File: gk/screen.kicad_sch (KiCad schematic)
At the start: 8 parts, among them J3 Conn_02x27_Top_Bottom, U5 PT4110E89E

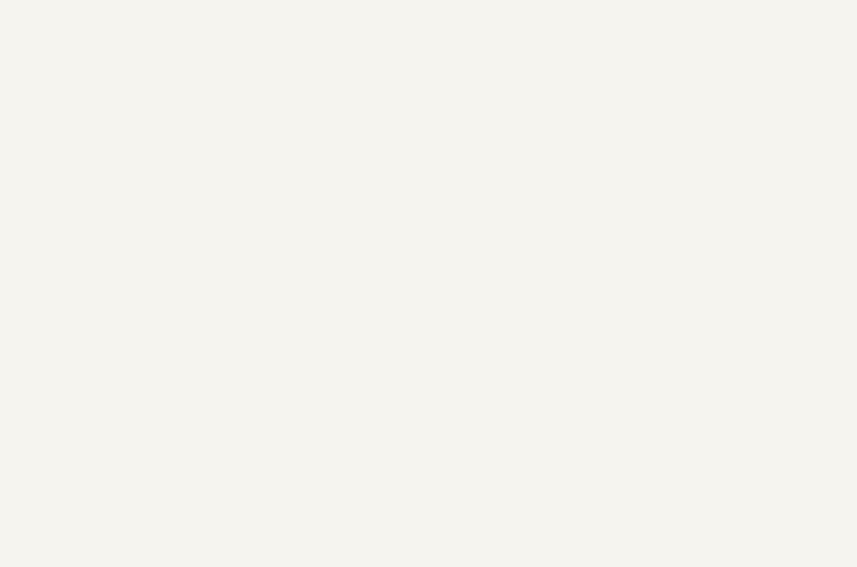
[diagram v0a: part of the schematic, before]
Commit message: Update pcb
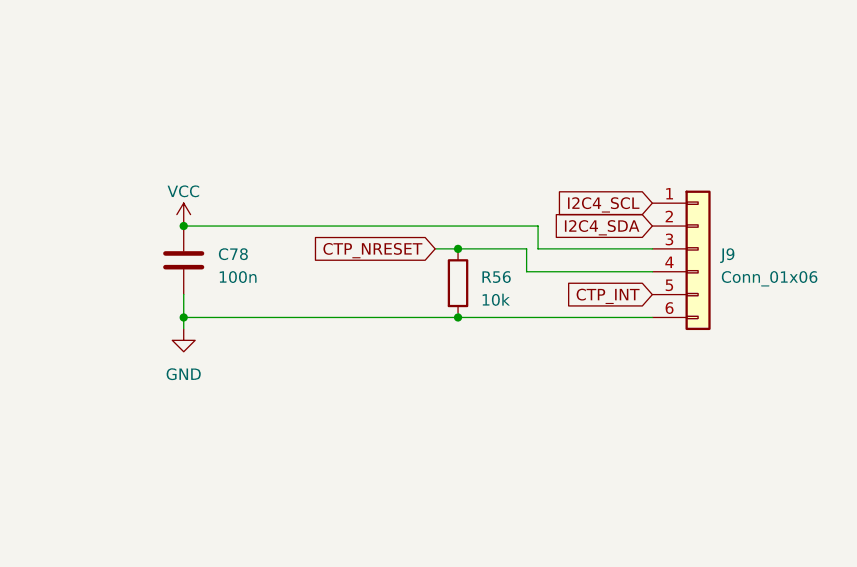
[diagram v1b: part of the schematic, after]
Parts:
- added C78: 100n, Capacitor_SMD:C_0603_1608Metric, symbol Device:C
- added J9: Conn_01x06, Connector_FFC-FPC:TE_0-1734839-6_1x06-1MP_P0.5mm_Horizontal, symbol Connector_Generic:Conn_01x06
- added R56: 10k, Resistor_SMD:R_0603_1608Metric, symbol Device:R
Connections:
- net GND: now also C78.2, J9.6 (Pin_6), R56.2
- net VCC: now also C78.1, J9.3 (Pin_3)
- new net CTP_INT: J9.5 (Pin_5)
- new net CTP_NRESET: J9.4 (Pin_4), R56.1
- new net I2C4_SCL: J9.1 (Pin_1)
- new net I2C4_SDA: J9.2 (Pin_2)
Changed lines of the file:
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@@
   (junction (at 105.41 54.61) (diameter 0) (color 0 0 0 0)
   )
+  (junction (at 179.07 52.07) (diameter 0) (color 0 0 0 0)
+  )
   (junction (at 140.97 82.55) (diameter 0) (color 0 0 0 0)
   )
@@
   (junction (at 63.5 58.42) (diameter 0) (color 0 0 0 0)
   )
+  (junction (at 209.55 62.23) (diameter 0) (color 0 0 0 0)
+  )
   (junction (at 86.36 48.26) (diameter 0) (color 0 0 0 0)
   )
@@
   (junction (at 88.9 60.96) (diameter 0) (color 0 0 0 0)
   )
+  (junction (at 179.07 62.23) (diameter 0) (color 0 0 0 0)
+  )
   (junction (at 46.99 58.42) (diameter 0) (color 0 0 0 0)
+  )
+  (junction (at 209.55 54.61) (diameter 0) (color 0 0 0 0)
   )
   (no_connect (at 134.62 102.87))
@@
     (stroke (width 0) (type default))
   )
+  (wire (pts (xy 209.55 62.23) (xy 231.14 62.23))
+    (stroke (width 0) (type default))
+  )
   (wire (pts (xy 73.66 69.85) (xy 73.66 67.31))
     (stroke (width 0) (type default))
@@
     (stroke (width 0) (type default))
   )
+  (wire (pts (xy 217.17 54.61) (xy 217.17 57.15))
+    (stroke (width 0) (type default))
+  )
+  (wire (pts (xy 207.01 54.61) (xy 209.55 54.61))
+    (stroke (width 0) (type default))
+  )
   (wire (pts (xy 105.41 48.26) (xy 105.41 54.61))
     (stroke (width 0) (type default))
@@
     (stroke (width 0) (type default))
   )
+  (wire (pts (xy 179.07 62.23) (xy 179.07 59.69))
+    (stroke (width 0) (type default))
+  )
   (wire (pts (xy 82.55 58.42) (xy 86.36 58.42))
     (stroke (width 0) (type default))
@@
     (stroke (width 0) (type default))
   )
+  (wire (pts (xy 179.07 63.5) (xy 179.07 62.23))
+    (stroke (width 0) (type default))
+  )
   (wire (pts (xy 105.41 54.61) (xy 116.84 54.61))
     (stroke (width 0) (type default))
@@
     (stroke (width 0) (type default))
   )
+  (wire (pts (xy 218.44 54.61) (xy 218.44 52.07))
+    (stroke (width 0) (type default))
+  )
   (wire (pts (xy 121.92 49.53) (xy 116.84 49.53))
     (stroke (width 0) (type default))
@@
     (stroke (width 0) (type default))
   )
+  (wire (pts (xy 218.44 52.07) (xy 179.07 52.07))
+    (stroke (width 0) (type default))
+  )
   (wire (pts (xy 60.96 69.85) (xy 73.66 69.85))
     (stroke (width 0) (type default))
@@
     (stroke (width 0) (type default))
   )
+  (wire (pts (xy 231.14 54.61) (xy 218.44 54.61))
+    (stroke (width 0) (type default))
+  )
   (wire (pts (xy 46.99 58.42) (xy 63.5 58.42))
     (stroke (width 0) (type default))
@@
     (stroke (width 0) (type default))
   )
+  (wire (pts (xy 217.17 57.15) (xy 231.14 57.15))
+    (stroke (width 0) (type default))
+  )
   (wire (pts (xy 134.62 115.57) (xy 137.16 115.57))
     (stroke (width 0) (type default))
@@
     (stroke (width 0) (type default))
   )
+  (wire (pts (xy 179.07 62.23) (xy 209.55 62.23))
+    (stroke (width 0) (type default))
+  )
   (wire (pts (xy 63.5 58.42) (xy 64.77 58.42))
     (stroke (width 0) (type default))
   )
+  (wire (pts (xy 209.55 54.61) (xy 217.17 54.61))
+    (stroke (width 0) (type default))
+  )
   (wire (pts (xy 105.41 54.61) (xy 99.06 54.61))
     (stroke (width 0) (type default))
@@
     )
   )
+  (global_label "I2C4_SCL" (shape input) (at 231.14 49.53 180) (fields_autoplaced)
+    (effects (font (size 1.27 1.27)) (justify right))
+    (property "Intersheetrefs" "${INTERSHEET_REFS}" (at 219.4652 49.53 0)
+      (effects (font (size 1.27 1.27)) (justify right) hide)
+    )
+  )
   (global_label "LTDC_R0" (shape input) (at 134.62 49.53 0) (fields_autoplaced)
     (effects (font (size 1.27 1.27)) (justify left))
@@
     )
   )
+  (global_label "CTP_NRESET" (shape input) (at 207.01 54.61 180) (fields_autoplaced)
+    (effects (font (size 1.27 1.27)) (justify right))
+    (property "Intersheetrefs" "${INTERSHEET_REFS}" (at 192.5534 54.61 0)
+      (effects (font (size 1.27 1.27)) (justify right) hide)
+    )
+  )
   (global_label "LTDC_R2" (shape input) (at 134.62 54.61 0) (fields_autoplaced)
     (effects (font (size 1.27 1.27)) (justify left))
@@
     )
   )
+  (global_label "I2C4_SDA" (shape input) (at 231.14 52.07 180) (fields_autoplaced)
+    (effects (font (size 1.27 1.27)) (justify right))
+    (property "Intersheetrefs" "${INTERSHEET_REFS}" (at 219.4047 52.07 0)
+      (effects (font (size 1.27 1.27)) (justify right) hide)
+    )
+  )
+  (global_label "CTP_INT" (shape input) (at 231.14 59.69 180) (fields_autoplaced)
+    (effects (font (size 1.27 1.27)) (justify right))
+    (property "Intersheetrefs" "${INTERSHEET_REFS}" (at 220.8561 59.69 0)
+      (effects (font (size 1.27 1.27)) (justify right) hide)
+    )
+  )
   (global_label "LTDC_G5" (shape input) (at 121.92 110.49 180) (fields_autoplaced)
     (effects (font (size 1.27 1.27)) (justify right))
@@
     (property "Intersheetrefs" "${INTERSHEET_REFS}" (at 111.0314 87.63 0)
       (effects (font (size 1.27 1.27)) (justify right) hide)
+    )
+  )
+  (symbol (lib_id "Device:C") (at 179.07 55.88 0) (unit 1)
+    (in_bom yes) (on_board yes) (dnp no) (fields_autoplaced)
+    (property "Reference" "C78" (at 182.88 55.245 0)
+      (effects (font (size 1.27 1.27)) (justify left))
+    )
+    (property "Value" "100n" (at 182.88 57.785 0)
+      (effects (font (size 1.27 1.27)) (justify left))
+    )
+    (property "Footprint" "Capacitor_SMD:C_0603_1608Metric" (at 180.0352 59.69 0)
+      (effects (font (size 1.27 1.27)) hide)
+    )
+    (property "Datasheet" "~" (at 179.07 55.88 0)
+      (effects (font (size 1.27 1.27)) hide)
+    )
+    (pin "1")
+    (pin "2")
+    (instances
+      (project "gk"
+        (path "/08730ac6-6084-459f-bdf1-86b322355ede/d5be4181-38f9-47fc-b63f-d0d72c8d11e3"
+          (reference "C78") (unit 1)
+        )
+      )
     )
   )
@@
     )
   )
+  (symbol (lib_id "Connector_Generic:Conn_01x06") (at 236.22 54.61 0) (unit 1)
+    (in_bom yes) (on_board yes) (dnp no) (fields_autoplaced)
+    (property "Reference" "J9" (at 238.76 55.245 0)
+      (effects (font (size 1.27 1.27)) (justify left))
+    )
+    (property "Value" "Conn_01x06" (at 238.76 57.785 0)
+      (effects (font (size 1.27 1.27)) (justify left))
+    )
+    (property "Footprint" "Connector_FFC-FPC:TE_0-1734839-6_1x06-1MP_P0.5mm_Horizontal" (at 236.22 54.61 0)
+      (effects (font (size 1.27 1.27)) hide)
+    )
+    (property "Datasheet" "~" (at 236.22 54.61 0)
+      (effects (font (size 1.27 1.27)) hide)
+    )
+    (pin "1")
+    (pin "2")
+    (pin "3")
+    (pin "4")
+    (pin "5")
+    (pin "6")
+    (instances
+      (project "gk"
+        (path "/08730ac6-6084-459f-bdf1-86b322355ede/d5be4181-38f9-47fc-b63f-d0d72c8d11e3"
+          (reference "J9") (unit 1)
+        )
+      )
+    )
+  )
   (symbol (lib_id "power:GND") (at 137.16 116.84 0) (unit 1)
     (in_bom yes) (on_board yes) (dnp no) (fields_autoplaced)
@@
         )
       )
+    )
+  )
+  (symbol (lib_id "Device:R") (at 209.55 58.42 0) (unit 1)
+    (in_bom yes) (on_board yes) (dnp no) (fields_autoplaced)
+    (property "Reference" "R56" (at 212.09 57.785 0)
+      (effects (font (size 1.27 1.27)) (justify left))
+    )
+    (property "Value" "10k" (at 212.09 60.325 0)
+      (effects (font (size 1.27 1.27)) (justify left))
+    )
+    (property "Footprint" "Resistor_SMD:R_0603_1608Metric" (at 207.772 58.42 90)
+      (effects (font (size 1.27 1.27)) hide)
+    )
+    (property "Datasheet" "~" (at 209.55 58.42 0)
+      (effects (font (size 1.27 1.27)) hide)
+    )
+    (pin "1")
+    (pin "2")
+    (instances
+      (project "gk"
+        (path "/08730ac6-6084-459f-bdf1-86b322355ede/d5be4181-38f9-47fc-b63f-d0d72c8d11e3"
+          (reference "R56") (unit 1)
+        )
+      )
+    )
+  )
+  (symbol (lib_id "power:GND") (at 179.07 63.5 0) (unit 1)
+    (in_bom yes) (on_board yes) (dnp no) (fields_autoplaced)
+    (property "Reference" "#PWR068" (at 179.07 69.85 0)
+      (effects (font (size 1.27 1.27)) hide)
+    )
+    (property "Value" "GND" (at 179.07 68.58 0)
+      (effects (font (size 1.27 1.27)))
+    )
+    (property "Footprint" "" (at 179.07 63.5 0)
+      (effects (font (size 1.27 1.27)) hide)
+    )
+    (property "Datasheet" "" (at 179.07 63.5 0)
+      (effects (font (size 1.27 1.27)) hide)
+    )
+    (pin "1")
+    (instances
+      (project "gk"
+        (path "/08730ac6-6084-459f-bdf1-86b322355ede/d5be4181-38f9-47fc-b63f-d0d72c8d11e3"
+          (reference "#PWR068") (unit 1)
+        )
+      )
+    )
+  )
+  (symbol (lib_id "power:VCC") (at 179.07 52.07 0) (unit 1)
+    (in_bom yes) (on_board yes) (dnp no) (fields_autoplaced)
+    (property "Reference" "#PWR067" (at 179.07 55.88 0)
+      (effects (font (size 1.27 1.27)) hide)
+    )
+    (property "Value" "VCC" (at 179.07 48.26 0)
+      (effects (font (size 1.27 1.27)))
+    )
+    (property "Footprint" "" (at 179.07 52.07 0)
+      (effects (font (size 1.27 1.27)) hide)
+    )
+    (property "Datasheet" "" (at 179.07 52.07 0)
+      (effects (font (size 1.27 1.27)) hide)
+    )
+    (pin "1")
+    (instances
+      (project "gk"
+        (path "/08730ac6-6084-459f-bdf1-86b322355ede/d5be4181-38f9-47fc-b63f-d0d72c8d11e3"
+          (reference "#PWR067") (unit 1)
+        )
+      )
